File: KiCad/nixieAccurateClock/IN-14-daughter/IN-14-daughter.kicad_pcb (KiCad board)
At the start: 4 copper layers, 19 x 32 mm, 9 parts, among them J1 Conn_02x05_Odd_Even, U1 HV509K6-G

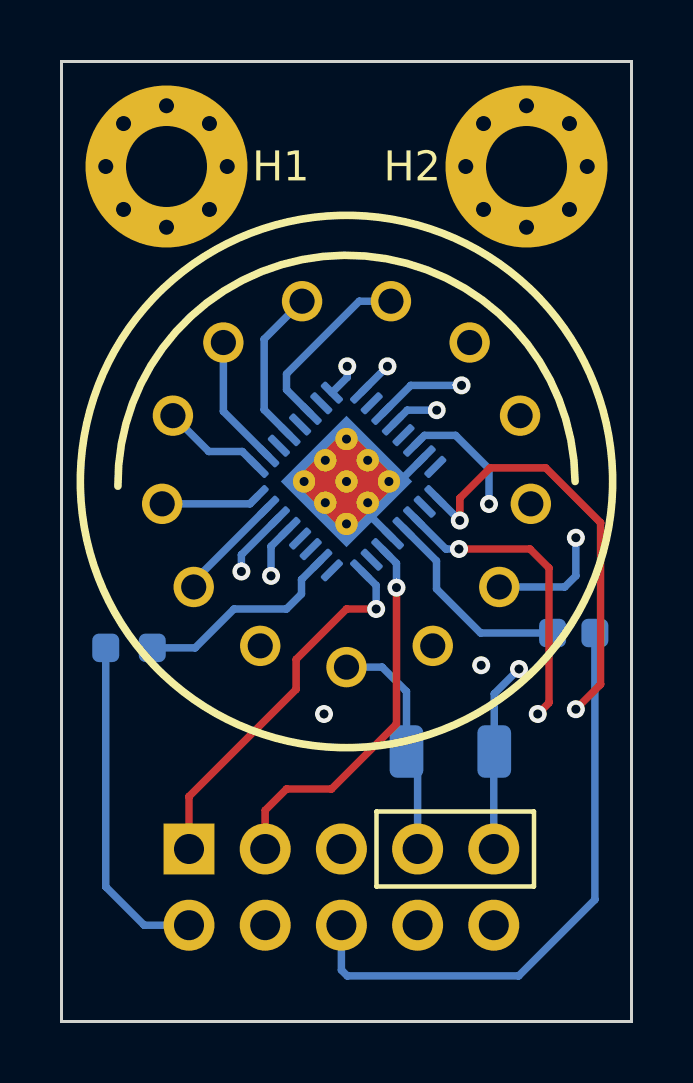
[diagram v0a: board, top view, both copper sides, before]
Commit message: add pin assignments
Pin assignment spreadsheet added
IN-14 daughter board traces smoothed
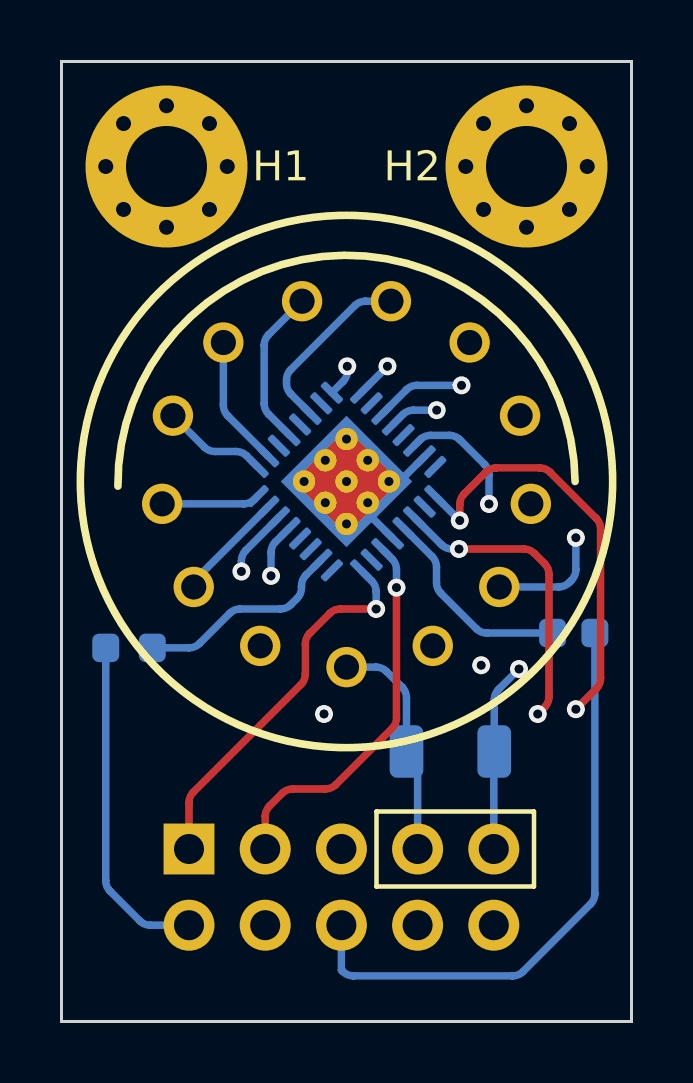
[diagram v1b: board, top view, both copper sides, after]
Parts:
- moved REF** 0.72 mm to (16.5, 26.0)
